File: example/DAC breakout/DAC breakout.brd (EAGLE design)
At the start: 35.5 x 17.4 mm, 8 parts, among them U1 MCP4822-E/P

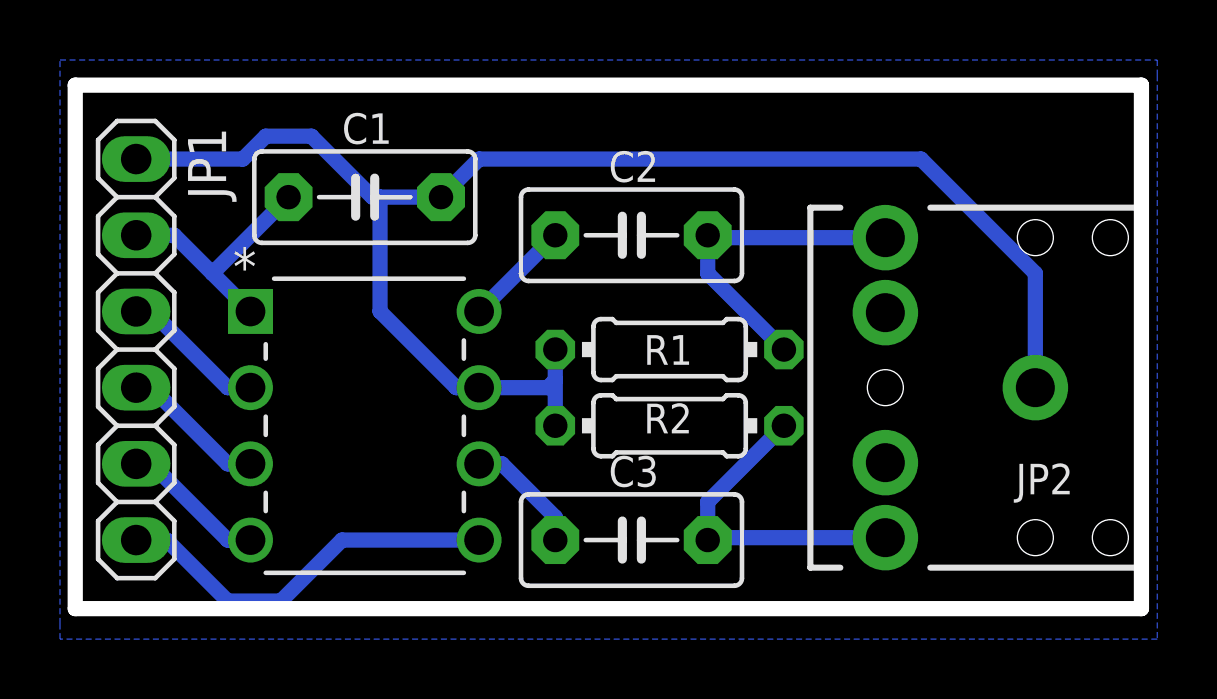
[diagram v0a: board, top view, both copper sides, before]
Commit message: added project files
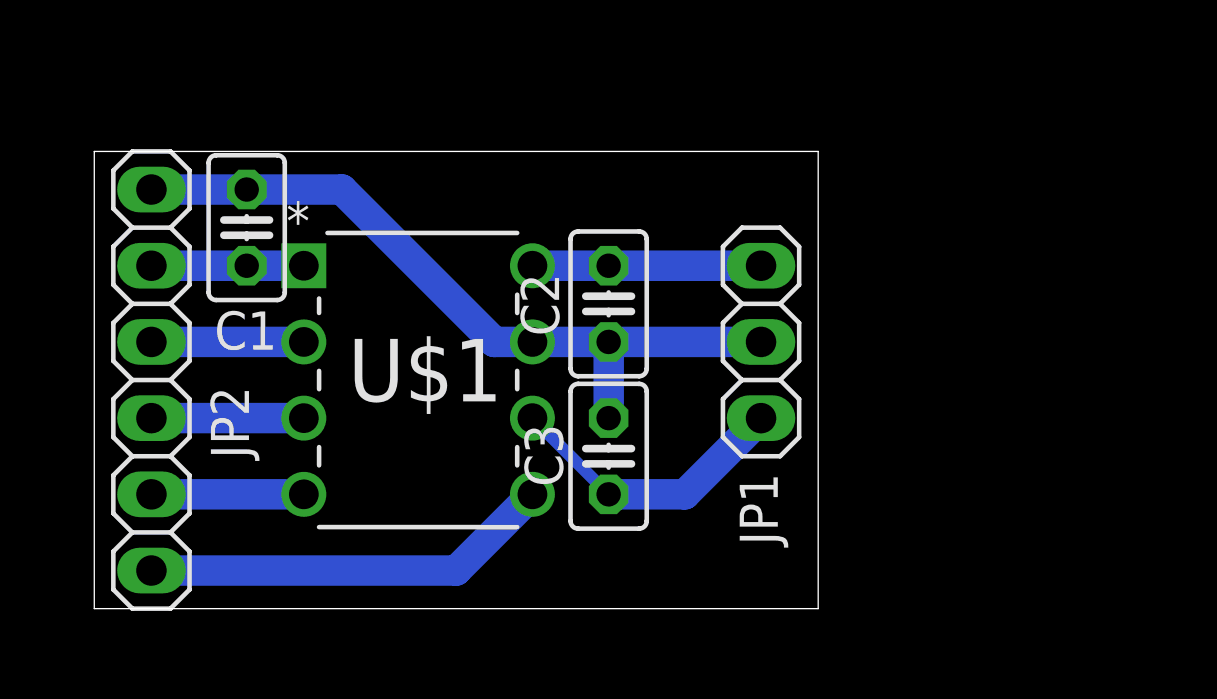
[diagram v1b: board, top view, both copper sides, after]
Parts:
- removed R1, R2: (no value), resistor:0204/7
- removed U1: MCP4822-E/P, Microchip_By_element14_Batch_1:DIP254P762X432-8
- added U$1: MCP4822-E/P, Microchip_By_element14_Batch_1:DIP254P762X432-8
- C1: value (none) -> 0.1uF; device capacitor-wima:C5B3 -> rcl:C025-025X050
- C2, C3: value (none) -> 1uF; device capacitor-wima:C5B3 -> rcl:C025-025X050
- JP1: device pinhead:1X06 -> pinhead:1X03
- JP2: device SparkFun-Connectors:AUDIO-JACK -> pinhead:1X06
- moved JP2 29.5 mm to (2.54, 7.62), turned to 90 degrees
- moved JP1 20.8 mm to (22.9, 8.89), turned to 270 degrees
- moved C1 4.07 mm to (5.71, 12.7), turned to 90 degrees
- moved C3 2.90 mm to (17.8, 5.08), turned to 90 degrees
- moved C2 2.41 mm to (17.8, 10.2), turned to 270 degrees
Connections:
- removed net N$8: C3.1, U1.6
- removed net N$9: C2.2, JP2.TIP, R1.1
- net GND: now also C2.2, C3.2, JP1.2, JP2.6, U$1.7; no longer JP1.6, JP2.SLEEVE, R1.2, R2.2, U1.7
- net N$1: now also C1.1, JP2.5, U$1.1; no longer JP1.1, U1.5
- net N$2: now also C2.1, JP1.1, U$1.8; no longer JP1.2, U1.4
- net N$3: now also C3.1, U$1.6; no longer U1.3
- net N$4: now also JP2.4, U$1.2; no longer JP1.4, U1.2
- net N$5: now also JP2.3, U$1.3; no longer C1.1, JP1.5, U1.1
- net N$6: now also JP2.2, U$1.4; no longer C3.2, JP2.RING, R2.1
- net N$7: now also JP2.1, U$1.5; no longer C2.1, U1.8
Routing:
- net GND: track 50.4 -> 25.0 mm
- net N$9: track 10.9 -> 0.00 mm
- net N$7: track 3.59 -> 13.8 mm
- net N$1: track 13.1 -> 5.08 mm
- net N$6: track 10.9 -> 5.08 mm
- net N$3: track 4.86 -> 9.72 mm
- net N$8: track 4.04 -> 0.00 mm
- net N$5: track 8.45 -> 5.08 mm
- net N$2: track 4.86 -> 7.62 mm
- removed copper zone on layer 16, net GND
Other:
- board size 35.5 x 17.4 mm -> 24.1 x 15.2 mm
